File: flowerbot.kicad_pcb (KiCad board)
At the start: 2 copper layers, 50 x 50 mm, 42 parts, among them P2 CONN_01X02, P3 CONN_01X03, P4 CONN_01X05, P5 USB_OTG, P7 CONN_01X02, U1 LM2937_3.3V, U2 ESP-07v2, U3 CP2102, U4 74LVC1G53

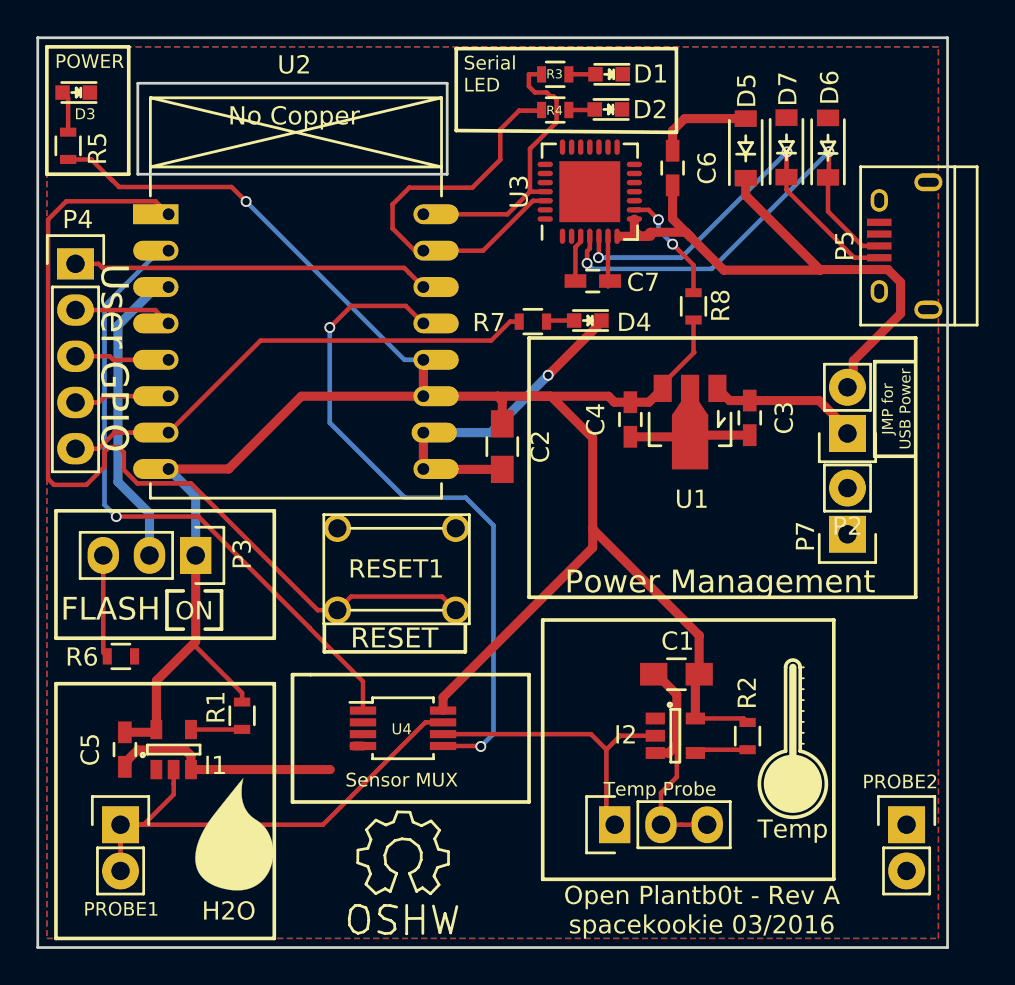
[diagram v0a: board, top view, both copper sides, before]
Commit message: Adding lots of gerber files, some new pictures, etc.
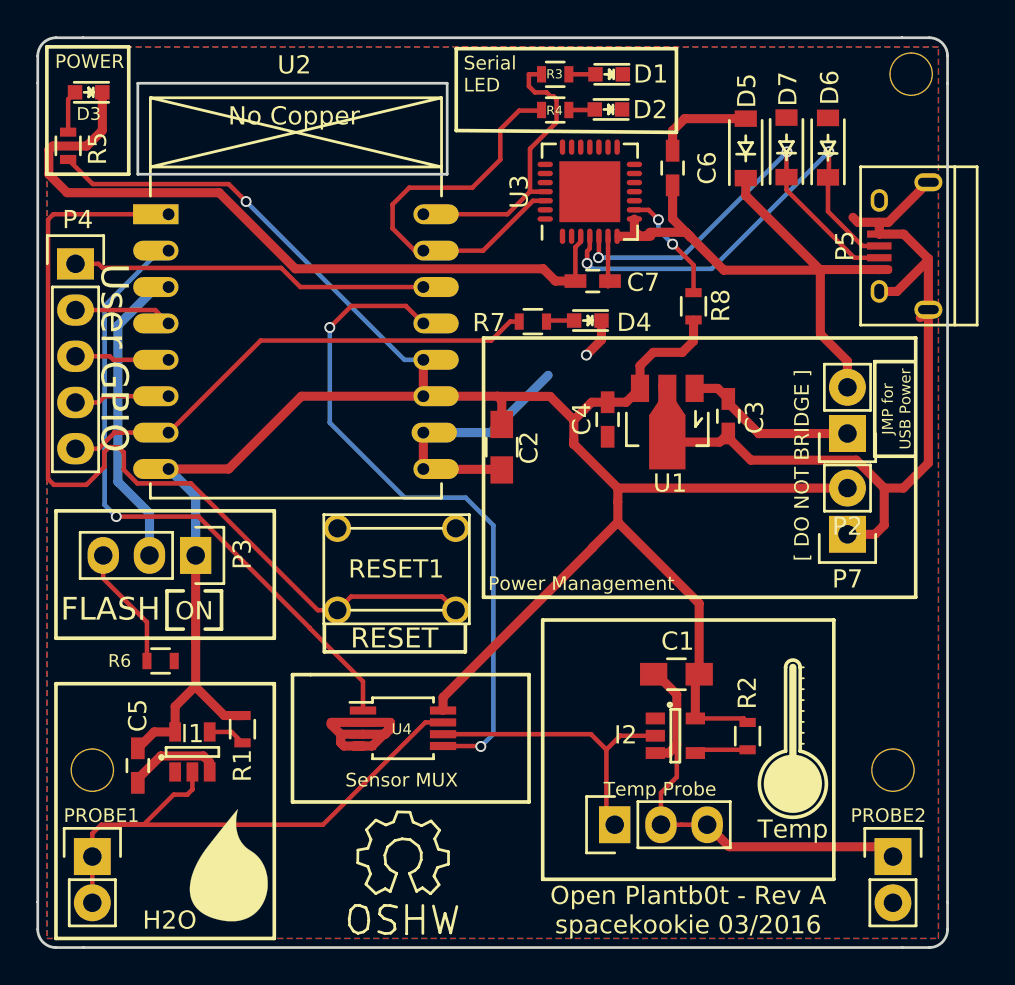
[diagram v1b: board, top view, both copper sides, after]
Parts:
- removed the G*** at (187.5, 59.3)
- added REF**: gnd_hole_2.25mm, kookie_utilities:gnd_hole_2.25mm, F.Cu at (153.0, 90.2)
- added REF**: gnd_hole_2.25mm, kookie_utilities:gnd_hole_2.25mm, F.Cu at (197.0, 90.2)
- added REF**: gnd_hole_2.25mm, kookie_utilities:gnd_hole_2.25mm, F.Cu at (198.0, 52.0)
- moved PROBE1 2.34 mm to (153.0, 95.0)
- moved R6 2.19 mm to (156.8, 84.2)
- moved PROBE2 1.90 mm to (197.0, 95.0)
- moved ? 1.73 mm to (160.5, 95.5)
- moved C4 1.25 mm to (181.3, 71.0), turned to 270 degrees
- moved U1 1.25 mm to (184.6, 71.1)
- moved C3 1.18 mm to (187.9, 70.8), turned to 90 degrees
- moved C5 1.13 mm to (155.5, 90.0)
- moved I1 1.04 mm to (158.5, 89.2)
- moved R1 0.74 mm to (161.2, 88.0)
- moved D3 0.69 mm to (152.8, 53.0)
- moved G*** 0.50 mm to (191.5, 92.0)
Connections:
- net /CURR_PROBE renamed /PROBE_SEL
- C3 pad 1: Net-(C3-Pad1) -> GND
- C3 pad 2: GND -> Net-(C3-Pad2)
- C4 pad 1: GND -> +3V3
- C4 pad 2: +3V3 -> GND
- P2 pad 1: Net-(C3-Pad1) -> Net-(C3-Pad2)
- P7 pad 2: (no net) -> +3V3
- U1 pad 1: Net-(C3-Pad1) -> Net-(C3-Pad2)
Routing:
- net GND: track 59.9 -> 149.2 mm
- net +3V3: track 122.2 -> 133.3 mm
- net Net-(C3-Pad2): track 0.00 -> 9.85 mm
- net Net-(C3-Pad1): track 8.47 -> 0.00 mm
- net /H2O_PROBE: track 27.6 -> 31.3 mm
- net Net-(P3-Pad3): track 5.64 -> 6.79 mm
- net Net-(I1-Pad4): track 2.81 -> 2.05 mm
- net +5V: track 35.2 -> 34.5 mm
- net /RES: track 50.4 -> 49.8 mm
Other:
- outline, holes or cut-outs redrawn
- board text added: "Programmer"
- board text added: "[ DO NOT BRIDGE ]"
- board text added: "https://github.com/spacekookie/open_plantb0t"
- board text removed: "github.com/spacekookie/open_plantb0t"
